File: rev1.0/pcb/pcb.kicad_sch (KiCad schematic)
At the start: 15 parts, among them J1 AVR-ISP-6, SW1 SW_Push, U1 ATMEGA32U4, Y1 16MHz

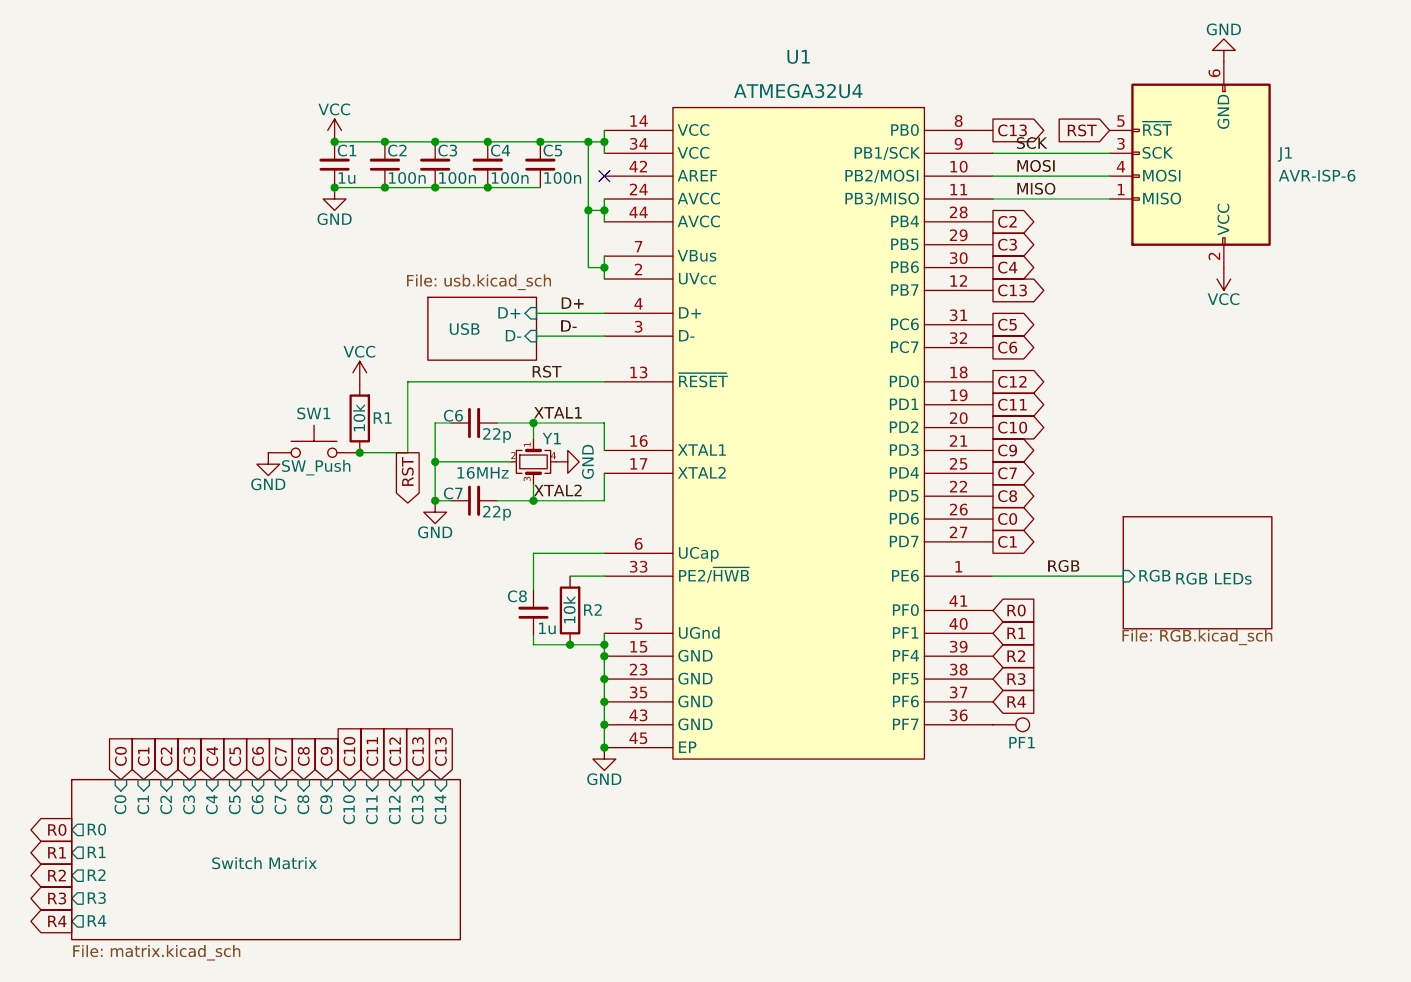
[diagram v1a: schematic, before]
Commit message: edited schematic and fixed constraints
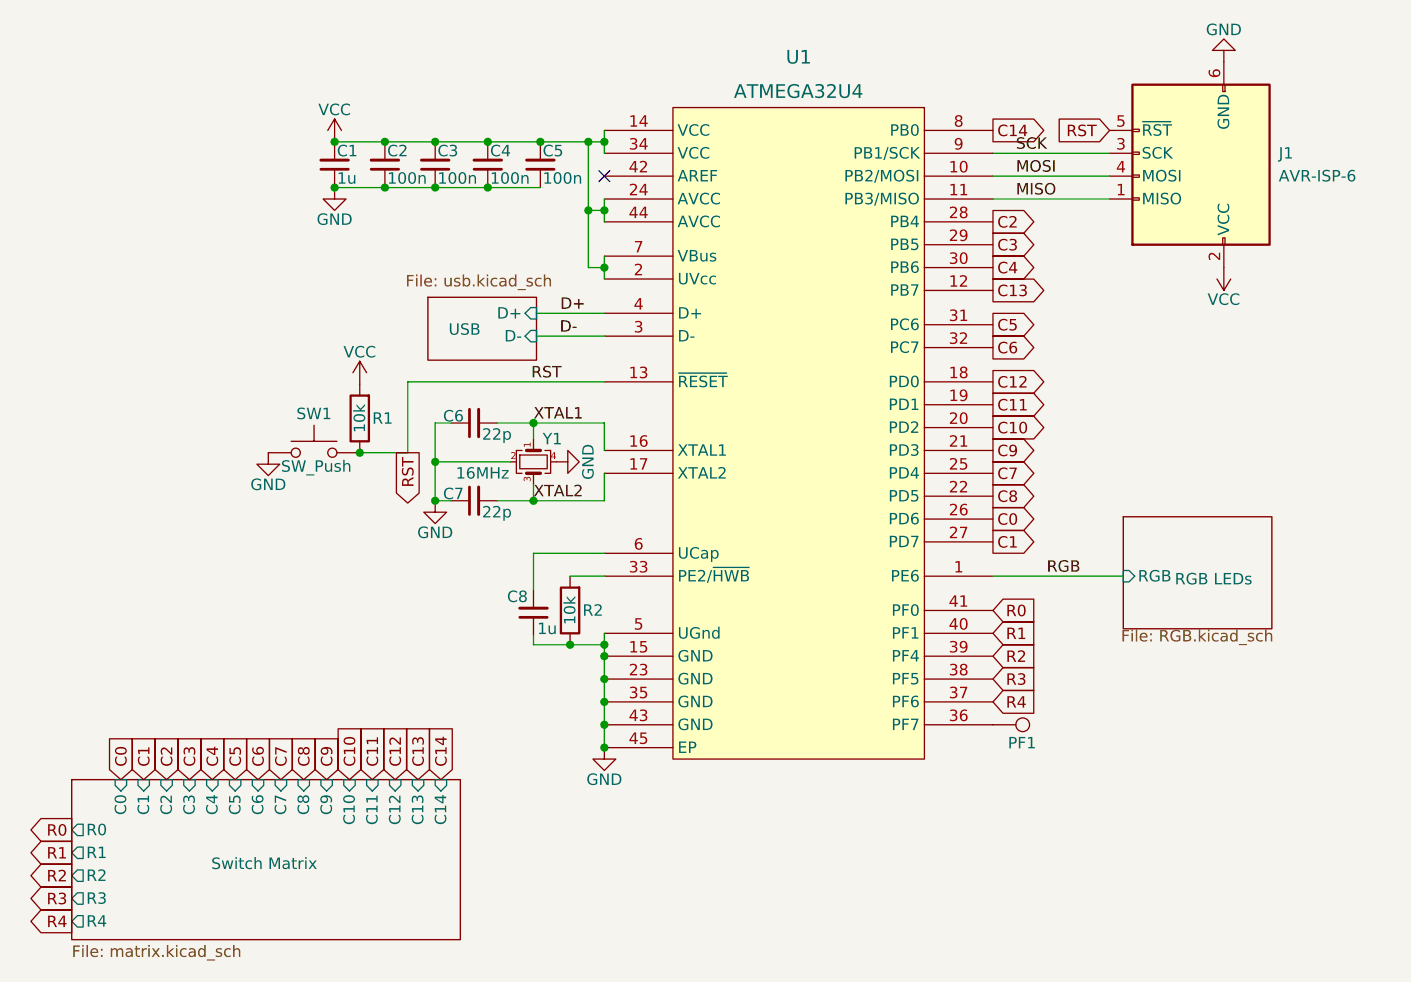
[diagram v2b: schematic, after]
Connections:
- net C13: no longer U1.8 (PB0)
- new net C14: U1.8 (PB0)
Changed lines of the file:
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@@
     )
   )
-  (global_label "C13" (shape input) (at 71.247 98.933 90) (fields_autoplaced)
-    (effects (font (size 1.27 1.27)) (justify left))
-    (property "Intersheet References" "${INTERSHEET_REFS}" (id 0) (at 71.1676 92.9262 90)
-      (effects (font (size 1.27 1.27)) (justify left) hide)
-    )
-  )
-  (global_label "C13" (shape output) (at 132.588 26.797 0) (fields_autoplaced)
+  (global_label "C14" (shape input) (at 71.247 98.933 90) (fields_autoplaced)
+    (effects (font (size 1.27 1.27)) (justify left))
+    (property "Intersheet References" "${INTERSHEET_REFS}" (id 0) (at 71.1676 92.8309 90)
+      (effects (font (size 1.27 1.27)) (justify left) hide)
+    )
+  )
+  (global_label "C14" (shape output) (at 132.588 26.797 0) (fields_autoplaced)
     (effects (font (size 1.27 1.27)) (justify left))
     (property "Intersheet References" "${INTERSHEET_REFS}" (id 0) (at 138.6901 26.7176 0)
@@
       (reference "D105") (unit 1) (value "BAV70") (footprint "Package_TO_SOT_SMD:SOT-23")
     )
-    (path "/c056f861-82ba-4a7e-9e72-5a4604669845/5439674f-83a9-4d9d-a767-d7965bd85a2f"
+    (path "/c056f861-82ba-4a7e-9e72-5a4604669845/f348a20a-82b1-4b09-af59-876b371d737b"
       (reference "D106") (unit 1) (value "BAV70") (footprint "Package_TO_SOT_SMD:SOT-23")
     )
-    (path "/c056f861-82ba-4a7e-9e72-5a4604669845/f348a20a-82b1-4b09-af59-876b371d737b"
+    (path "/c056f861-82ba-4a7e-9e72-5a4604669845/155a85ab-0052-4faa-b39d-826485ce9896"
       (reference "D107") (unit 1) (value "BAV70") (footprint "Package_TO_SOT_SMD:SOT-23")
     )
-    (path "/c056f861-82ba-4a7e-9e72-5a4604669845/155a85ab-0052-4faa-b39d-826485ce9896"
+    (path "/c056f861-82ba-4a7e-9e72-5a4604669845/e8ff04d5-920b-441f-8472-dbeb2358c0d7"
       (reference "D108") (unit 1) (value "BAV70") (footprint "Package_TO_SOT_SMD:SOT-23")
     )
-    (path "/c056f861-82ba-4a7e-9e72-5a4604669845/e8ff04d5-920b-441f-8472-dbeb2358c0d7"
+    (path "/c056f861-82ba-4a7e-9e72-5a4604669845/06ba327d-1471-4837-8194-dff19381ed4d"
       (reference "D109") (unit 1) (value "BAV70") (footprint "Package_TO_SOT_SMD:SOT-23")
     )
-    (path "/c056f861-82ba-4a7e-9e72-5a4604669845/06ba327d-1471-4837-8194-dff19381ed4d"
+    (path "/c056f861-82ba-4a7e-9e72-5a4604669845/f27ee04c-0530-4e51-a49b-bbc414265e15"
       (reference "D110") (unit 1) (value "BAV70") (footprint "Package_TO_SOT_SMD:SOT-23")
     )
-    (path "/c056f861-82ba-4a7e-9e72-5a4604669845/f27ee04c-0530-4e51-a49b-bbc414265e15"
+    (path "/c056f861-82ba-4a7e-9e72-5a4604669845/667d98ff-975e-4b44-87d4-965528898ffe"
       (reference "D111") (unit 1) (value "BAV70") (footprint "Package_TO_SOT_SMD:SOT-23")
     )
-    (path "/c056f861-82ba-4a7e-9e72-5a4604669845/667d98ff-975e-4b44-87d4-965528898ffe"
+    (path "/c056f861-82ba-4a7e-9e72-5a4604669845/eb396c18-f4cd-492d-ab4f-a0ada45298d5"
       (reference "D112") (unit 1) (value "BAV70") (footprint "Package_TO_SOT_SMD:SOT-23")
     )
-    (path "/c056f861-82ba-4a7e-9e72-5a4604669845/eb396c18-f4cd-492d-ab4f-a0ada45298d5"
+    (path "/c056f861-82ba-4a7e-9e72-5a4604669845/1a0eeafb-71b2-45f0-9e0d-009dc92a7cfe"
       (reference "D113") (unit 1) (value "BAV70") (footprint "Package_TO_SOT_SMD:SOT-23")
     )
-    (path "/c056f861-82ba-4a7e-9e72-5a4604669845/1a0eeafb-71b2-45f0-9e0d-009dc92a7cfe"
+    (path "/c056f861-82ba-4a7e-9e72-5a4604669845/2231c462-b6bb-43b1-a0d7-d4017e3f4feb"
       (reference "D114") (unit 1) (value "BAV70") (footprint "Package_TO_SOT_SMD:SOT-23")
     )
-    (path "/c056f861-82ba-4a7e-9e72-5a4604669845/2231c462-b6bb-43b1-a0d7-d4017e3f4feb"
+    (path "/c056f861-82ba-4a7e-9e72-5a4604669845/dd6a311b-d698-4f9a-9cda-b74981dd28b8"
       (reference "D115") (unit 1) (value "BAV70") (footprint "Package_TO_SOT_SMD:SOT-23")
     )
-    (path "/c056f861-82ba-4a7e-9e72-5a4604669845/dd6a311b-d698-4f9a-9cda-b74981dd28b8"
+    (path "/c056f861-82ba-4a7e-9e72-5a4604669845/43512e93-857c-42a1-9d3f-e16a44d77df2"
       (reference "D116") (unit 1) (value "BAV70") (footprint "Package_TO_SOT_SMD:SOT-23")
     )
-    (path "/c056f861-82ba-4a7e-9e72-5a4604669845/43512e93-857c-42a1-9d3f-e16a44d77df2"
+    (path "/c056f861-82ba-4a7e-9e72-5a4604669845/94c3c277-42e6-434c-84f3-116e945148bf"
       (reference "D117") (unit 1) (value "BAV70") (footprint "Package_TO_SOT_SMD:SOT-23")
     )
-    (path "/c056f861-82ba-4a7e-9e72-5a4604669845/94c3c277-42e6-434c-84f3-116e945148bf"
+    (path "/c056f861-82ba-4a7e-9e72-5a4604669845/4c67f2b5-10dc-4c73-aa28-c77bb571f6d2"
       (reference "D118") (unit 1) (value "BAV70") (footprint "Package_TO_SOT_SMD:SOT-23")
     )
-    (path "/c056f861-82ba-4a7e-9e72-5a4604669845/4c67f2b5-10dc-4c73-aa28-c77bb571f6d2"
+    (path "/c056f861-82ba-4a7e-9e72-5a4604669845/e17b61f2-97db-49a7-8fbc-9d7490ea5114"
       (reference "D119") (unit 1) (value "BAV70") (footprint "Package_TO_SOT_SMD:SOT-23")
     )
-    (path "/c056f861-82ba-4a7e-9e72-5a4604669845/e17b61f2-97db-49a7-8fbc-9d7490ea5114"
-      (reference "D120") (unit 1) (value "BAV70") (footprint "Package_TO_SOT_SMD:SOT-23")
-    )
     (path "/3ee7a193-1c79-43da-aa5f-923bdb6badb0/d11caa8e-0735-474f-86fc-57561ca10317"
-      (reference "D121") (unit 1) (value "SMF5.0CA") (footprint "Diode_SMD:D_SOD-123F")
+      (reference "D120") (unit 1) (value "SMF5.0CA") (footprint "Diode_SMD:D_SOD-123F")
     )
     (path "/3ee7a193-1c79-43da-aa5f-923bdb6badb0/85c9a0c5-f049-48b6-9560-e81ad0b53bcb"
@@
     )
     (path "/3ee7a193-1c79-43da-aa5f-923bdb6badb0/92fc67ca-dfa2-4746-9284-02d5c226cc5d"
-      (reference "J2") (unit 1) (value "USB4120-03-C") (footprint "0xcb:MOLEX_2130830005")
+      (reference "J2") (unit 1) (value "USB4120-03-C") (footprint "0xcb:GCT_USB4105_REVA")
     )
     (path "/c056f861-82ba-4a7e-9e72-5a4604669845/57b2c139-70ea-4a57-b03c-a17b8cbc199a"

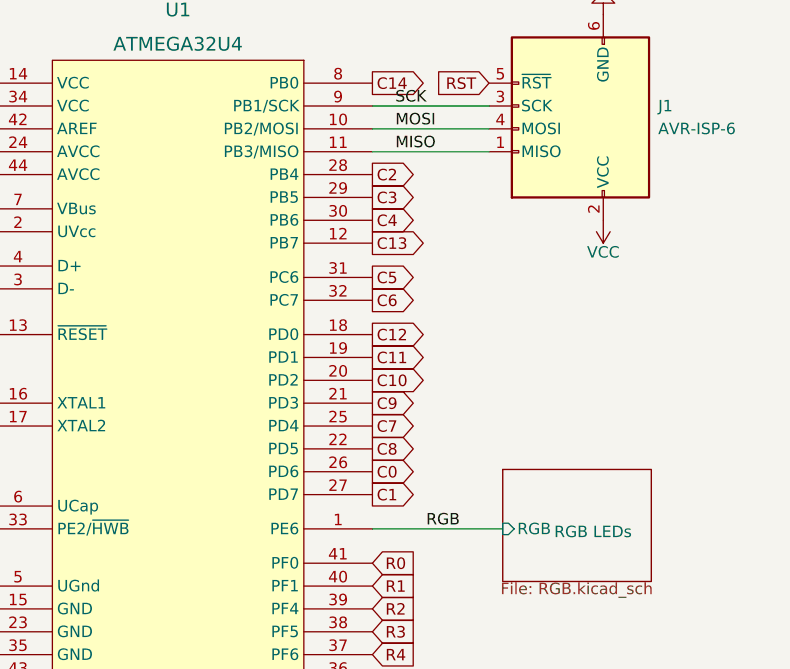
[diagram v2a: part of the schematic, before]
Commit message: Did some columns and rows to controller
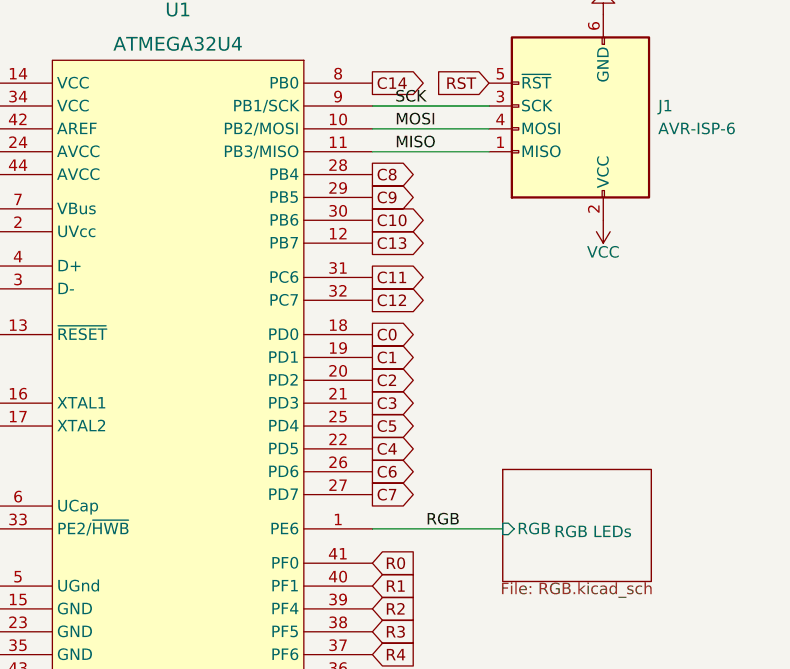
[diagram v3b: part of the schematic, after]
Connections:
- net C0: now also U1.18 (PD0); no longer U1.26 (PD6)
- net C1: now also U1.19 (PD1); no longer U1.27 (PD7)
- net C10: now also U1.30 (PB6); no longer U1.20 (PD2)
- net C11: now also U1.31 (PC6); no longer U1.19 (PD1)
- net C12: now also U1.32 (PC7); no longer U1.18 (PD0)
- net C2: now also U1.20 (PD2); no longer U1.28 (PB4)
- net C3: now also U1.21 (PD3); no longer U1.29 (PB5)
- net C4: now also U1.22 (PD5); no longer U1.30 (PB6)
- net C5: now also U1.25 (PD4); no longer U1.31 (PC6)
- net C6: now also U1.26 (PD6); no longer U1.32 (PC7)
- net C7: now also U1.27 (PD7); no longer U1.25 (PD4)
- net C8: now also U1.28 (PB4); no longer U1.22 (PD5)
- net C9: now also U1.29 (PB5); no longer U1.21 (PD3)
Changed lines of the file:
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@@
     )
   )
-  (global_label "C2" (shape output) (at 132.588 36.957 0) (fields_autoplaced)
+  (global_label "C8" (shape output) (at 132.588 36.957 0) (fields_autoplaced)
     (effects (font (size 1.27 1.27)) (justify left))
     (property "Intersheet References" "${INTERSHEET_REFS}" (id 0) (at 137.3853 36.8776 0)
@@
     )
   )
-  (global_label "C3" (shape output) (at 132.588 39.497 0) (fields_autoplaced)
+  (global_label "C9" (shape output) (at 132.588 39.497 0) (fields_autoplaced)
     (effects (font (size 1.27 1.27)) (justify left))
     (property "Intersheet References" "${INTERSHEET_REFS}" (id 0) (at 137.3853 39.4176 0)
@@
     )
   )
-  (global_label "C4" (shape output) (at 132.588 42.037 0) (fields_autoplaced)
+  (global_label "C10" (shape output) (at 132.588 42.037 0) (fields_autoplaced)
     (effects (font (size 1.27 1.27)) (justify left))
-    (property "Intersheet References" "${INTERSHEET_REFS}" (id 0) (at 137.3853 41.9576 0)
+    (property "Intersheet References" "${INTERSHEET_REFS}" (id 0) (at 138.5948 41.9576 0)
       (effects (font (size 1.27 1.27)) (justify left) hide)
     )
@@
     )
   )
-  (global_label "C5" (shape output) (at 132.588 48.387 0) (fields_autoplaced)
+  (global_label "C11" (shape output) (at 132.588 48.387 0) (fields_autoplaced)
     (effects (font (size 1.27 1.27)) (justify left))
-    (property "Intersheet References" "${INTERSHEET_REFS}" (id 0) (at 137.3853 48.3076 0)
+    (property "Intersheet References" "${INTERSHEET_REFS}" (id 0) (at 138.5948 48.3076 0)
       (effects (font (size 1.27 1.27)) (justify left) hide)
     )
   )
-  (global_label "C6" (shape output) (at 132.588 50.927 0) (fields_autoplaced)
+  (global_label "C12" (shape output) (at 132.588 50.927 0) (fields_autoplaced)
     (effects (font (size 1.27 1.27)) (justify left))
-    (property "Intersheet References" "${INTERSHEET_REFS}" (id 0) (at 137.3853 50.8476 0)
+    (property "Intersheet References" "${INTERSHEET_REFS}" (id 0) (at 138.5948 50.8476 0)
       (effects (font (size 1.27 1.27)) (justify left) hide)
     )
   )
-  (global_label "C12" (shape output) (at 132.588 54.737 0) (fields_autoplaced)
+  (global_label "C0" (shape output) (at 132.588 54.737 0) (fields_autoplaced)
     (effects (font (size 1.27 1.27)) (justify left))
-    (property "Intersheet References" "${INTERSHEET_REFS}" (id 0) (at 138.5948 54.6576 0)
+    (property "Intersheet References" "${INTERSHEET_REFS}" (id 0) (at 137.3853 54.6576 0)
       (effects (font (size 1.27 1.27)) (justify left) hide)
     )
   )
-  (global_label "C11" (shape output) (at 132.588 57.277 0) (fields_autoplaced)
+  (global_label "C1" (shape output) (at 132.588 57.277 0) (fields_autoplaced)
     (effects (font (size 1.27 1.27)) (justify left))
-    (property "Intersheet References" "${INTERSHEET_REFS}" (id 0) (at 138.5948 57.1976 0)
+    (property "Intersheet References" "${INTERSHEET_REFS}" (id 0) (at 137.3853 57.1976 0)
       (effects (font (size 1.27 1.27)) (justify left) hide)
     )
   )
-  (global_label "C10" (shape output) (at 132.588 59.817 0) (fields_autoplaced)
+  (global_label "C2" (shape output) (at 132.588 59.817 0) (fields_autoplaced)
     (effects (font (size 1.27 1.27)) (justify left))
-    (property "Intersheet References" "${INTERSHEET_REFS}" (id 0) (at 138.5948 59.7376 0)
+    (property "Intersheet References" "${INTERSHEET_REFS}" (id 0) (at 137.3853 59.7376 0)
       (effects (font (size 1.27 1.27)) (justify left) hide)
     )
   )
-  (global_label "C9" (shape output) (at 132.588 62.357 0) (fields_autoplaced)
+  (global_label "C3" (shape output) (at 132.588 62.357 0) (fields_autoplaced)
     (effects (font (size 1.27 1.27)) (justify left))
     (property "Intersheet References" "${INTERSHEET_REFS}" (id 0) (at 137.3853 62.2776 0)
@@
     )
   )
-  (global_label "C7" (shape output) (at 132.588 64.897 0) (fields_autoplaced)
+  (global_label "C5" (shape output) (at 132.588 64.897 0) (fields_autoplaced)
     (effects (font (size 1.27 1.27)) (justify left))
     (property "Intersheet References" "${INTERSHEET_REFS}" (id 0) (at 137.3853 64.8176 0)
@@
     )
   )
-  (global_label "C8" (shape output) (at 132.588 67.437 0) (fields_autoplaced)
+  (global_label "C4" (shape output) (at 132.588 67.437 0) (fields_autoplaced)
     (effects (font (size 1.27 1.27)) (justify left))
     (property "Intersheet References" "${INTERSHEET_REFS}" (id 0) (at 137.3853 67.3576 0)
@@
     )
   )
-  (global_label "C0" (shape output) (at 132.588 69.977 0) (fields_autoplaced)
+  (global_label "C6" (shape output) (at 132.588 69.977 0) (fields_autoplaced)
     (effects (font (size 1.27 1.27)) (justify left))
     (property "Intersheet References" "${INTERSHEET_REFS}" (id 0) (at 137.3853 69.8976 0)
@@
     )
   )
-  (global_label "C1" (shape output) (at 132.588 72.517 0) (fields_autoplaced)
+  (global_label "C7" (shape output) (at 132.588 72.517 0) (fields_autoplaced)
     (effects (font (size 1.27 1.27)) (justify left))
     (property "Intersheet References" "${INTERSHEET_REFS}" (id 0) (at 137.3853 72.4376 0)
